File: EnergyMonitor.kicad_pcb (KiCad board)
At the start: 2 copper layers, 100 x 140 mm, 131 parts, among them J1 IN, J2 OUT, J3 V, J4 UART, J5 Conn_01x06, J6 5V, J7 3V3, Q1 2N3906, U1 BD4830G, U10 LNK3202P, U11 AMS1117-3.3, U12 MCP39F501, U13 74LVC1G14, U14 PC817, U2 MCP9700AT-ETT, U3 74LVC1G14, U4 74LVC1G14, U5 PC827, U6 PC817, U7 PC817, U8 PC817, U9 TL431DBZ, X1 SG-310, Y1 4MHz

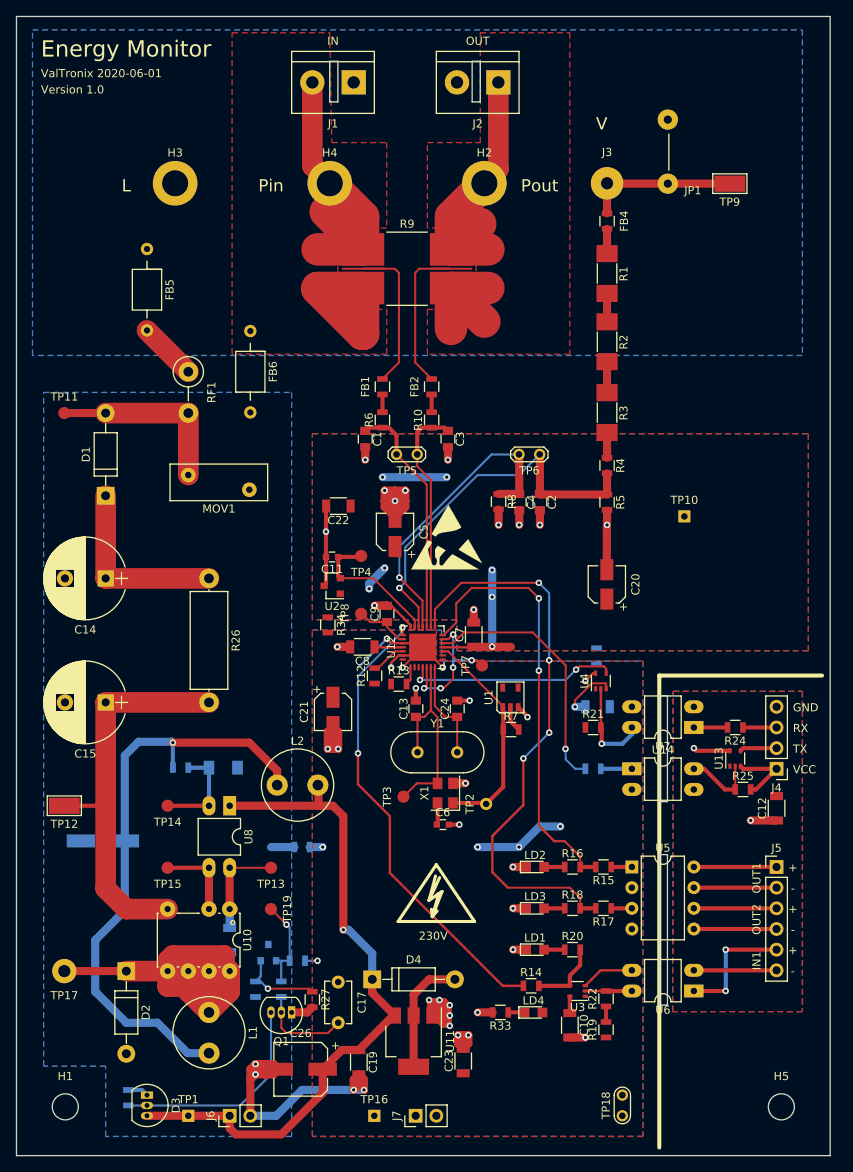
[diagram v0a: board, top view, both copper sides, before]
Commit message: Routage
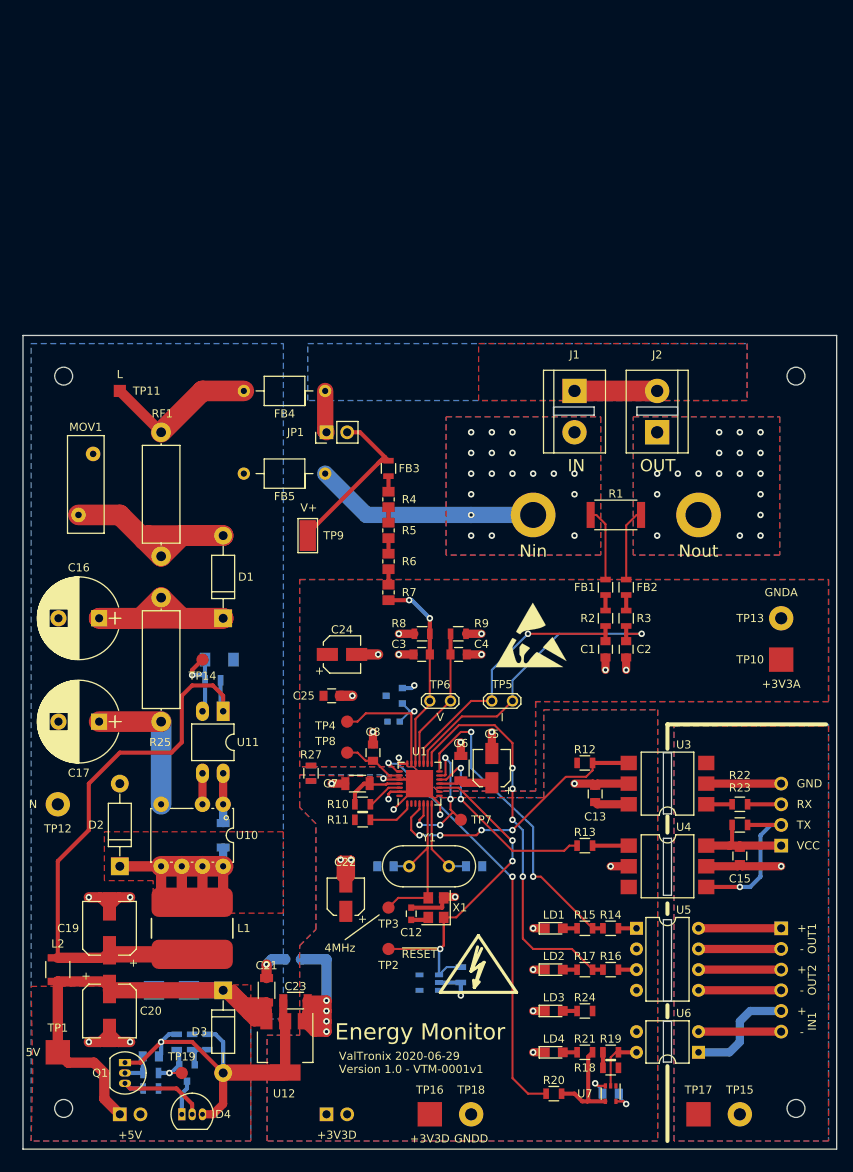
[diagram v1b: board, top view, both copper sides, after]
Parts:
- removed the C10 at (118.0, 154.0)
- removed the C12 at (143.4, 127.3)
- removed the C25 at (121.4, 114.8)
- removed the C26 at (84.9, 159.4)
- removed the C9 at (95.5, 103.4)
- removed the FB4 at (122.6, 55.1)
- removed the H1 at (56.0, 164.0)
- removed J3: V, Wire_Pads:SolderWirePad_single_1-5mmDrill
- removed the R1 at (122.6, 61.6)
- removed the R2 at (122.6, 70.0)
- removed the R25 at (139.3, 125.0)
- removed the R33 at (109.5, 152.4)
- removed the U12 at (99.9, 107.5)
- removed the U13 at (138.3, 121.2)
- removed U14: PC817, ValTronix:DIP-4_W7.62mm_LongPads
- added C13: 100nF, ValTronix:C_0805, F.Cu at (121.1, 125.5)
- added C15: 100nF, ValTronix:C_0805, F.Cu at (138.9, 133.2)
- added C16: 4.7µF, ValTronix:CP_Radial_D10.0mm_P5.00mm, F.Cu at (60.2, 104.0)
- added C20: 47µF, ValTronix:CP_Elec_6.3x7.7, F.Cu at (61.4, 152.2)
- added C8: 100nF, ValTronix:C_0805, F.Cu at (93.8, 120.5)
- added D5: SMBJ5.0A, ValTronix:D_SMB, B.Cu at (69.0, 149.7)
- added FB3: BLM18PG121SN1D, ValTronix:L_0805, F.Cu at (95.7, 85.5)
- added H4: M2, Mounting_Holes:MountingHole_2.2mm_M2_ISO14580, F.Cu at (145.8, 74.2)
- added H6: M2, Mounting_Holes:MountingHole_2.2mm_M2_ISO14580, F.Cu at (145.8, 164.2)
- added R10: 4.7k, ValTronix:R_0805, F.Cu at (92.5, 126.8)
- added R13: 1k, ValTronix:R_0805, F.Cu at (119.8, 131.9)
- added R5: 330k, ValTronix:R_MicroMELF_MMU-0102, F.Cu at (95.7, 93.2)
- added R7: 9.1k, ValTronix:R_MicroMELF_MMU-0102, F.Cu at (95.7, 100.8)
- added U1: MCP39F501, ValTronix:QFN-28-1EP_5x5mm_Pitch0.5mm, F.Cu at (99.5, 124.3)
- C10: renamed from C24; moved to B.Cu
- C11, J4, J5, J6, J7, U2: moved to B.Cu
- C14: value 6.8µF -> 100nF; footprint ValTronix:CP_Radial_D10.0mm_P5.00mm -> ValTronix:C_0805; moved to B.Cu
- C17: renamed from C15; value 6.8µF -> 4.7µF
- C19: renamed from C18; moved to F.Cu
- C25: renamed from C22; footprint ValTronix:C_1206 -> ValTronix:C_0805
- C26: renamed from C17; footprint ValTronix:C_Disc_D5.1mm_W3.2mm_P5.00mm -> ValTronix:C_0805; moved to B.Cu
- C9: renamed from C13; moved to B.Cu
- H1: renamed from H4; value N -> Nin
- H2: value Nload -> Nout
- H3: value L -> M2; footprint Mounting_Holes:MountingHole_3.2mm_M3_ISO14580_Pad -> Mounting_Holes:MountingHole_2.2mm_M2_ISO14580
- H5: value MountingHole -> M2; footprint Mounting_Holes:MountingHole_3.2mm_M3_ISO14580 -> Mounting_Holes:MountingHole_2.2mm_M2_ISO14580
- JP1: footprint Wire_Connections_Bridges:WireConnection_1.00mmDrill -> Pin_Headers:Pin_Header_Straight_1x02_Pitch2.54mm
- L1: value 2mH -> 1800µH; footprint ValTronix:L_Radial_D8.7mm_P5.00mm_Fastron_07HCP -> ValTronix:L_Bourns_SDR1006
- L2: footprint ValTronix:L_Radial_D8.7mm_P5.00mm_Fastron_07HCP -> ValTronix:L_1210
- R1: renamed from R9; footprint ValTronix:R_Shunt_8.75x5.6mm -> ValTronix:R_2512
- R12: value 4.7k -> 1k
- R14: value 200 -> 2k
- R15, R17: value 2k -> 1k
- R16: value 1k -> 2k
- R18: value 1k -> 10k
- R20: value 1k -> 200
- R21, R22: value 10k -> 1k
- R23: moved to F.Cu
- R28: renamed from R7; value 4.7k -> 33k; moved to B.Cu
- R29: renamed from R27; moved to B.Cu
- R4: value 9.1k -> 330k; footprint ValTronix:R_0805 -> ValTronix:R_MicroMELF_MMU-0102
- R6: renamed from R3; footprint ValTronix:R_MELF_MMB-0207 -> ValTronix:R_MicroMELF_MMU-0102
- RF1: footprint ValTronix:R_Axial_DIN0411_L9.9mm_D3.6mm_P5.08mm_Vertical -> ValTronix:R_Axial_DIN0414_L11.9mm_D4.5mm_P15.24mm_Horizontal
- SYM3: value 240V -> 230V
- TP1, TP10, TP16: footprint Measurement_Points:Measurement_Point_Square-TH_Small -> Measurement_Points:Measurement_Point_Square-SMD-Pad_Big
- TP11: value LRF -> L; footprint Measurement_Points:Measurement_Point_Round-SMD-Pad_Small -> Measurement_Points:Measurement_Point_Square-SMD-Pad_Small
- TP12: value D -> N; footprint Measurement_Points:Test_Point_Keystone_5019_Minature -> Measurement_Points:Measurement_Point_Round-TH_Big
- TP13: value BP -> GNDA; footprint Measurement_Points:Measurement_Point_Round-SMD-Pad_Small -> Measurement_Points:Measurement_Point_Round-TH_Big
- TP15: value FB -> GND; footprint Measurement_Points:Measurement_Point_Round-SMD-Pad_Small -> Measurement_Points:Measurement_Point_Round-TH_Big
- TP17: value S -> VCC; footprint Measurement_Points:Measurement_Point_Round-TH_Big -> Measurement_Points:Measurement_Point_Square-SMD-Pad_Big
- TP18: footprint Measurement_Points:Test_Point -> Measurement_Points:Measurement_Point_Round-TH_Big
- TP2: footprint Measurement_Points:Measurement_Point_Round-TH_Small -> Measurement_Points:Measurement_Point_Round-SMD-Pad_Small
- U13: renamed from U1; moved to B.Cu
- U3, U4: value 74LVC1G14 -> H11L1SM; footprint ValTronix:SOT-353_SC-70-5 -> ValTronix:SMDIP-6_W9.53mm
- U6: footprint ValTronix:DIP-4_W7.62mm_LongPads -> ValTronix:DIP-4_W7.62mm
- U7: value PC817 -> 74LVC1G14; footprint ValTronix:DIP-4_W7.62mm_LongPads -> ValTronix:SOT-353_SC-70-5
- moved SYM3 93.7 mm to (116.0, 157.3)
- moved C14 88.7 mm to (123.0, 162.4)
- moved H5 88.2 mm to (55.8, 164.2)
- moved TP17 79.9 mm to (133.8, 164.9), turned to 0 degrees
- moved TP15 76.6 mm to (138.9, 164.9), turned to 0 degrees
- moved TP13 69.8 mm to (144.0, 104.0), turned to 0 degrees
- moved TP9 67.5 mm to (85.8, 93.8), turned to 270 degrees
- moved JP1 50.1 mm to (88.1, 81.1), turned to 90 degrees
- moved H2 48.5 mm to (133.8, 91.3)
- moved H1 47.8 mm to (113.5, 91.3)
- moved J2 47.2 mm to (128.7, 81.1), turned to 90 degrees
- moved J1 46.6 mm to (118.6, 76.0), turned to 270 degrees
- moved U7 46.1 mm to (123.0, 162.4), turned to 270 degrees
- moved R21 39.9 mm to (119.8, 157.3)
- moved R1 39.7 mm to (123.7, 91.3)
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- renumbered C6 to C12, C16 to C18, C3 to C2, C19 to C21, C21 to C22, C20 to C24, C2 to C3, C7 to C6, C8 to C7, D4 to D3, D3 to D4, FB5 to FB4, FB6 to FB5, FB3 to FB6, R11 to NT1, R13 to R11, R6 to R2, R26 to R25, R32 to R26, R34 to R27, R10 to R3, R28 to R30, R29 to R31, R30 to R32, R31 to R33, R5 to R8, R8 to R9, U8 to U11, U11 to U12
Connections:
- C14 pad 1: /PSU 3V3 Referenced to mains/LCC -> +3V3
- C14 pad 2: /N -> GNDD
- C19 pad 1: Net-(C18-Pad1) -> /PSU 3V3 Referenced to mains/S+
- D4 pad 3: /PSU 3V3 Referenced to mains/5V -> +3V3
- FB1 pad 2: Net-(FB1-Pad2) -> /Nin
- FB2 pad 2: Net-(FB2-Pad2) -> /Nout
- H3 pad 1: /Lio -> (no net)
- L1 pad 2: Net-(C18-Pad1) -> /PSU 3V3 Referenced to mains/S+
- L2 pad 1: Net-(C18-Pad1) -> /PSU 3V3 Referenced to mains/S+
- LD1 pad 2: /DI3L -> /DO0L
- LD2 pad 2: /DO0L -> /DO1L
- LD3 pad 2: /DO1L -> Net-(LD3-Pad2)
- LD4 pad 1: Net-(LD4-Pad1) -> GNDD
- LD4 pad 2: +3V3 -> /DI3L
- R1 pad 2: Net-(FB1-Pad2) -> /Nout
- R12 pad 2: /~MCLR -> /RX_MON
- R14 pad 1: /DIO3 -> /DO0
- R14 pad 2: Net-(R14-Pad2) -> /DIO0
- R15 pad 1: /DO0 -> /DO0L
- R16 pad 1: /DO0L -> /DO1
- R16 pad 2: /DIO0 -> /DIO1
- R17 pad 1: /DO1 -> /DO1L
- R18 pad 1: /DO1L -> +3V3
- R18 pad 2: /DIO1 -> Net-(R18-Pad2)
- R19 pad 1: +3V3 -> Net-(R18-Pad2)
- R19 pad 2: Net-(R19-Pad2) -> /~DI3
- R20 pad 1: /DI3L -> /DIO3
- R20 pad 2: Net-(R14-Pad2) -> Net-(R20-Pad2)
- R21 pad 1: +3V3 -> /DI3L
- R21 pad 2: Net-(R21-Pad2) -> Net-(R20-Pad2)
- R22 pad 1: Net-(R19-Pad2) -> /RX
- R22 pad 2: /~DI3 -> Net-(R22-Pad2)
- R23 pad 1: Net-(R23-Pad1) -> /TX
- R23 pad 2: /TX_MON -> VCC
- R24 pad 1: /RX -> +3V3
- R24 pad 2: Net-(R24-Pad2) -> Net-(LD3-Pad2)
- R26 pad 1: Net-(C18-Pad1) -> /PSU 3V3 Referenced to mains/S+
- R4 pad 1: Net-(R3-Pad2) -> Net-(FB3-Pad2)
- R4 pad 2: /V1+ -> Net-(R4-Pad2)
- R6 pad 2: Net-(R3-Pad2) -> Net-(R6-Pad2)
- TP11 pad 1: /PSU 3V3 Referenced to mains/LRF -> /L
- TP12 pad 1: /PSU 3V3 Referenced to mains/D -> /N
- TP13 pad 1: /PSU 3V3 Referenced to mains/BP -> GNDA
- TP15 pad 1: /PSU 3V3 Referenced to mains/FB -> GND
- TP17 pad 1: /PSU 3V3 Referenced to mains/S -> VCC
- U11 pad 1: /PSU 3V3 Referenced to mains/5V -> /PSU 3V3 Referenced to mains/S+
- U3 pad 1: (no net) -> Net-(R22-Pad2)
- U3 pad 2: /~DI3 -> GND
- U3 pad 3: GNDD -> Net-(U3-Pad3)
- U3 pad 4: Net-(R14-Pad2) -> /RX_MON
- U3 pad 5: +3V3 -> GNDD
- U4 pad 1: (no net) -> Net-(R13-Pad1)
- U4 pad 2: Net-(R21-Pad2) -> GNDD
- U4 pad 3: +3V3 -> Net-(U4-Pad3)
- U4 pad 4: /RX_MON -> /TX
- U4 pad 5: GNDD -> GND
- U7 pad 1: Net-(R24-Pad2) -> (no net)
- U7 pad 2: GND -> /~DI3
- U7 pad 4: Net-(R21-Pad2) -> Net-(R20-Pad2)
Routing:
- net Net-(C18-Pad1): track 73.4 -> 0.00 mm, vias 1 -> 0
- net /PSU 3V3 Referenced to mains/S+: track 0.00 -> 71.3 mm
- net /Nout: track 47.9 -> 9.02 mm, vias 0 -> 18
- net GNDA: track 60.2 -> 22.3 mm
- net /PSU 3V3 Referenced to mains/S: track 64.7 -> 31.5 mm
- net /PSU 3V3 Referenced to mains/D: track 49.3 -> 17.8 mm
- net /N: track 44.9 -> 20.6 mm, vias 4 -> 5
- net /V1+: track 48.1 -> 24.6 mm, vias 1 -> 2
- net /DIO1: track 70.6 -> 49.6 mm
- net +3.3VA: track 29.0 -> 8.34 mm, vias 7 -> 1
- net +3V3: track 49.1 -> 69.7 mm, vias 5 -> 3
- net /PSU 3V3 Referenced to mains/5V: track 84.6 -> 64.2 mm, vias 1 -> 0
- net /V1-: track 37.9 -> 17.5 mm, vias 1 -> 0
- net Net-(FB2-Pad2): track 18.5 -> 0.00 mm
- net Net-(FB1-Pad2): track 18.5 -> 0.00 mm
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- added copper zone on F.Cu, net /Lio
- added copper zone on B.Cu, net /Nin
- added copper zone on B.Cu, net /Nout
- added copper zone on F.Cu, net /PSU 3V3 Referenced to mains/5V
- added copper zone on F.Cu, net /PSU 3V3 Referenced to mains/S
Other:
- board size 100 x 140 mm -> 100 x 100 mm
- board text added: "+3V3 and +5V are referenced to mains"
- board text added: "+3V3 or +5V"
- board text added: "+3V3D"
- board text added: "+5V"
- board text added: "Insolated area"
- board text added: "Nin"
- board text added: "Nout"
- board text added: "ValTronix 2020-06-29 Version 1.0 - VTM-0001v1"
- board text added: "WARNING! RISK OF ELECTRICAL SHOCK!"
- board text removed: "L"
- board text removed: "Pin"
- board text removed: "Pout"
- board text removed: "V"
- board text removed: "ValTronix 2020-06-01"
- board text removed: "Version 1.0"
